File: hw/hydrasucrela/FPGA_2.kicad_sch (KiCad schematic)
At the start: 1 part, among them U1 ECP5U_25_CABGA381

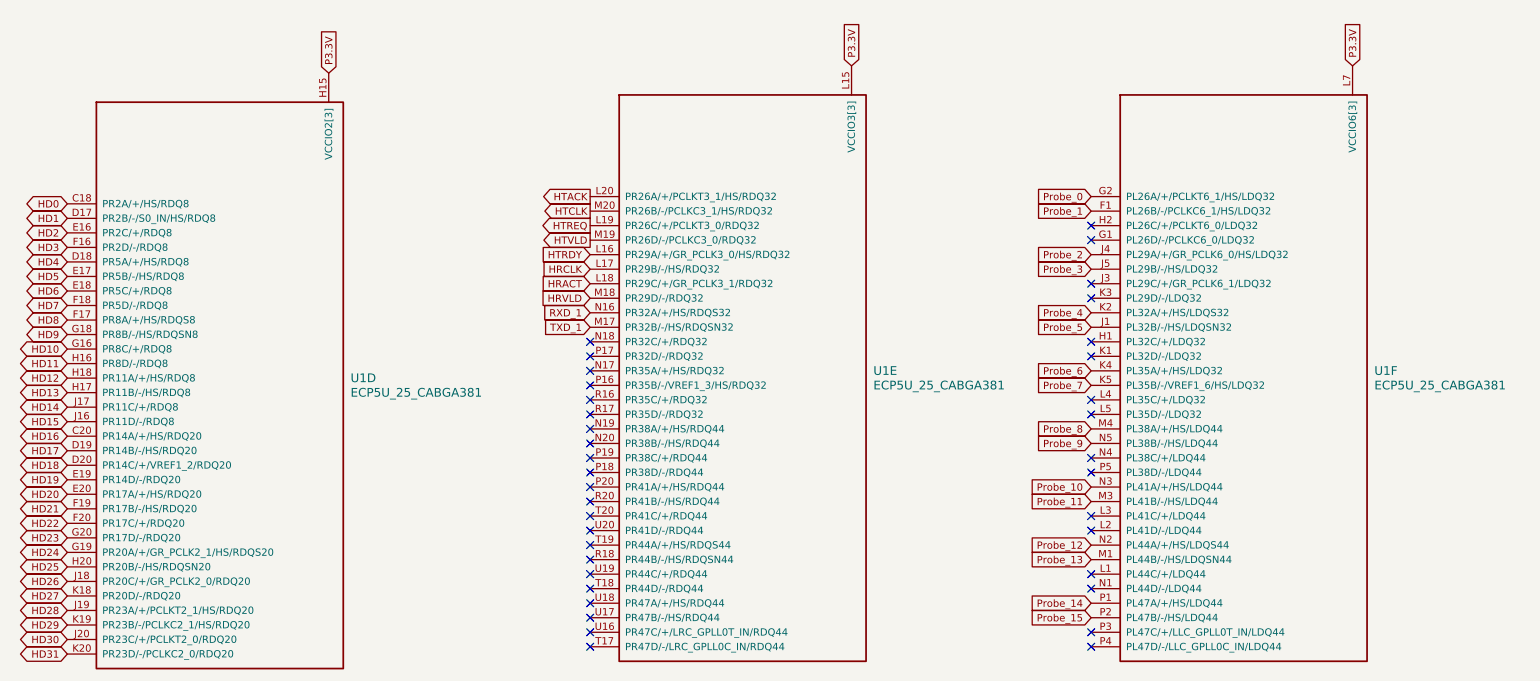
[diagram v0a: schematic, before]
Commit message: Update HydraSucreLA PCB
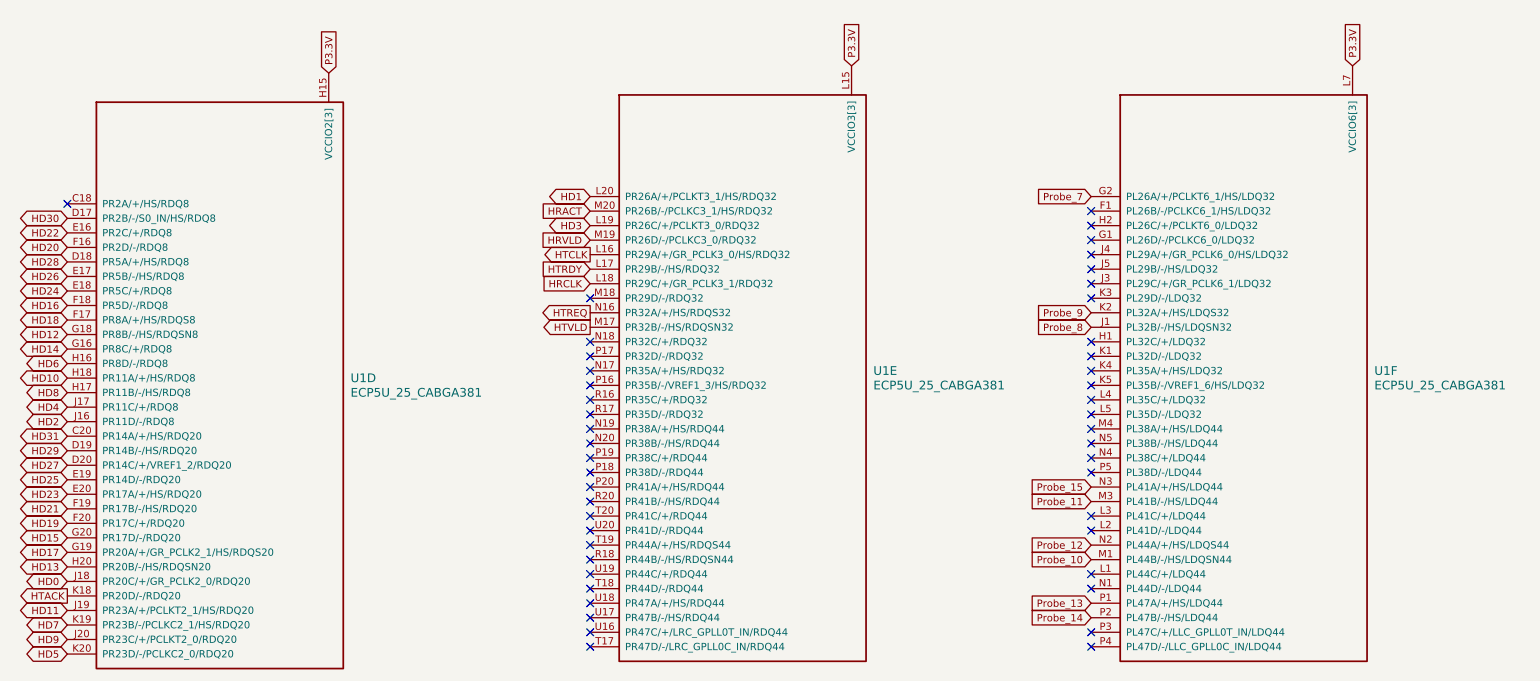
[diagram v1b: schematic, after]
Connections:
- net Probe_0 is gone; now on net Probe_7: U1.G2 (PL26A/+/PCLKT6_1/HS/LDQ32)
- net Probe_4 is gone; now on net Probe_9: U1.K2 (PL32A/+/HS/LDQS32)
- net Probe_5 is gone; now on net Probe_8: U1.J1 (PL32B/-/HS/LDQSN32)
- net RXD_1 is gone; now on net HTREQ: U1.N16 (PR32A/+/HS/RDQS32)
- net TXD_1 is gone; now on net HTVLD: U1.M17 (PR32B/-/HS/RDQSN32)
- net HD0: now also U1.J18 (PR20C/+/GR_PCLK2_0/RDQ20); no longer U1.C18 (PR2A/+/HS/RDQ8)
- net HD1: now also U1.L20 (PR26A/+/PCLKT3_1/HS/RDQ32); no longer U1.D17 (PR2B/-/S0_IN/HS/RDQ8)
- net HD10: now also U1.H18 (PR11A/+/HS/RDQ8); no longer U1.G16 (PR8C/+/RDQ8)
- net HD11: now also U1.J19 (PR23A/+/PCLKT2_1/HS/RDQ20); no longer U1.H16 (PR8D/-/RDQ8)
- net HD12: now also U1.G18 (PR8B/-/HS/RDQSN8); no longer U1.H18 (PR11A/+/HS/RDQ8)
- net HD13: now also U1.H20 (PR20B/-/HS/RDQSN20); no longer U1.H17 (PR11B/-/HS/RDQ8)
- net HD14: now also U1.G16 (PR8C/+/RDQ8); no longer U1.J17 (PR11C/+/RDQ8)
- net HD15: now also U1.G20 (PR17D/-/RDQ20); no longer U1.J16 (PR11D/-/RDQ8)
- net HD16: now also U1.F18 (PR5D/-/RDQ8); no longer U1.C20 (PR14A/+/HS/RDQ20)
- net HD17: now also U1.G19 (PR20A/+/GR_PCLK2_1/HS/RDQS20); no longer U1.D19 (PR14B/-/HS/RDQ20)
- net HD18: now also U1.F17 (PR8A/+/HS/RDQS8); no longer U1.D20 (PR14C/+/VREF1_2/RDQ20)
- net HD19: now also U1.F20 (PR17C/+/RDQ20); no longer U1.E19 (PR14D/-/RDQ20)
- net HD2: now also U1.J16 (PR11D/-/RDQ8); no longer U1.E16 (PR2C/+/RDQ8)
- net HD20: now also U1.F16 (PR2D/-/RDQ8); no longer U1.E20 (PR17A/+/HS/RDQ20)
- net HD22: now also U1.E16 (PR2C/+/RDQ8); no longer U1.F20 (PR17C/+/RDQ20)
- net HD23: now also U1.E20 (PR17A/+/HS/RDQ20); no longer U1.G20 (PR17D/-/RDQ20)
- net HD24: now also U1.E18 (PR5C/+/RDQ8); no longer U1.G19 (PR20A/+/GR_PCLK2_1/HS/RDQS20)
- net HD25: now also U1.E19 (PR14D/-/RDQ20); no longer U1.H20 (PR20B/-/HS/RDQSN20)
- net HD26: now also U1.E17 (PR5B/-/HS/RDQ8); no longer U1.J18 (PR20C/+/GR_PCLK2_0/RDQ20)
- net HD27: now also U1.D20 (PR14C/+/VREF1_2/RDQ20); no longer U1.K18 (PR20D/-/RDQ20)
- net HD28: now also U1.D18 (PR5A/+/HS/RDQ8); no longer U1.J19 (PR23A/+/PCLKT2_1/HS/RDQ20)
- net HD29: now also U1.D19 (PR14B/-/HS/RDQ20); no longer U1.K19 (PR23B/-/PCLKC2_1/HS/RDQ20)
- net HD3: now also U1.L19 (PR26C/+/PCLKT3_0/RDQ32); no longer U1.F16 (PR2D/-/RDQ8)
- net HD30: now also U1.D17 (PR2B/-/S0_IN/HS/RDQ8); no longer U1.J20 (PR23C/+/PCLKT2_0/RDQ20)
- net HD31: now also U1.C20 (PR14A/+/HS/RDQ20); no longer U1.K20 (PR23D/-/PCLKC2_0/RDQ20)
- net HD4: now also U1.J17 (PR11C/+/RDQ8); no longer U1.D18 (PR5A/+/HS/RDQ8)
- net HD5: now also U1.K20 (PR23D/-/PCLKC2_0/RDQ20); no longer U1.E17 (PR5B/-/HS/RDQ8)
- net HD6: now also U1.H16 (PR8D/-/RDQ8); no longer U1.E18 (PR5C/+/RDQ8)
- net HD7: now also U1.K19 (PR23B/-/PCLKC2_1/HS/RDQ20); no longer U1.F18 (PR5D/-/RDQ8)
- net HD8: now also U1.H17 (PR11B/-/HS/RDQ8); no longer U1.F17 (PR8A/+/HS/RDQS8)
- net HD9: now also U1.J20 (PR23C/+/PCLKT2_0/RDQ20); no longer U1.G18 (PR8B/-/HS/RDQSN8)
- net HRACT: now also U1.M20 (PR26B/-/PCLKC3_1/HS/RDQ32); no longer U1.L18 (PR29C/+/GR_PCLK3_1/RDQ32)
- net HRCLK: now also U1.L18 (PR29C/+/GR_PCLK3_1/RDQ32); no longer U1.L17 (PR29B/-/HS/RDQ32)
- net HRVLD: now also U1.M19 (PR26D/-/PCLKC3_0/RDQ32); no longer U1.M18 (PR29D/-/RDQ32)
- net HTACK: now also U1.K18 (PR20D/-/RDQ20); no longer U1.L20 (PR26A/+/PCLKT3_1/HS/RDQ32)
- net HTCLK: now also U1.L16 (PR29A/+/GR_PCLK3_0/HS/RDQ32); no longer U1.M20 (PR26B/-/PCLKC3_1/HS/RDQ32)
- net HTRDY: now also U1.L17 (PR29B/-/HS/RDQ32); no longer U1.L16 (PR29A/+/GR_PCLK3_0/HS/RDQ32)
- net HTREQ: no longer U1.L19 (PR26C/+/PCLKT3_0/RDQ32)
- net HTVLD: no longer U1.M19 (PR26D/-/PCLKC3_0/RDQ32)
- net Probe_10: now also U1.M1 (PL44B/-/HS/LDQSN44); no longer U1.N3 (PL41A/+/HS/LDQ44)
- net Probe_13: now also U1.P1 (PL47A/+/HS/LDQ44); no longer U1.M1 (PL44B/-/HS/LDQSN44)
- net Probe_14: now also U1.P2 (PL47B/-/HS/LDQ44); no longer U1.P1 (PL47A/+/HS/LDQ44)
- net Probe_15: now also U1.N3 (PL41A/+/HS/LDQ44); no longer U1.P2 (PL47B/-/HS/LDQ44)
- net Probe_7: no longer U1.K5 (PL35B/-/VREF1_6/HS/LDQ32)
- net Probe_8: no longer U1.M4 (PL38A/+/HS/LDQ44)
- net Probe_9: no longer U1.N5 (PL38B/-/HS/LDQ44)
- net Probe_1: no longer names the net of U1.F1 (PL26B/-/PCLKC6_1/HS/LDQ32)
- net Probe_2: no longer names the net of U1.J4 (PL29A/+/GR_PCLK6_0/HS/LDQ32)
- net Probe_3: no longer names the net of U1.J5 (PL29B/-/HS/LDQ32)
- net Probe_6: no longer names the net of U1.K4 (PL35A/+/HS/LDQ32)
- no-connect marks 38 -> 47
